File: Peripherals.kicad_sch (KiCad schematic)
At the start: 6 parts, among them J1 Conn_01x02, J4 Conn_02x10_Counter_Clockwise, Q1 PMOS, Q2 NMOS, U6 TPS62133

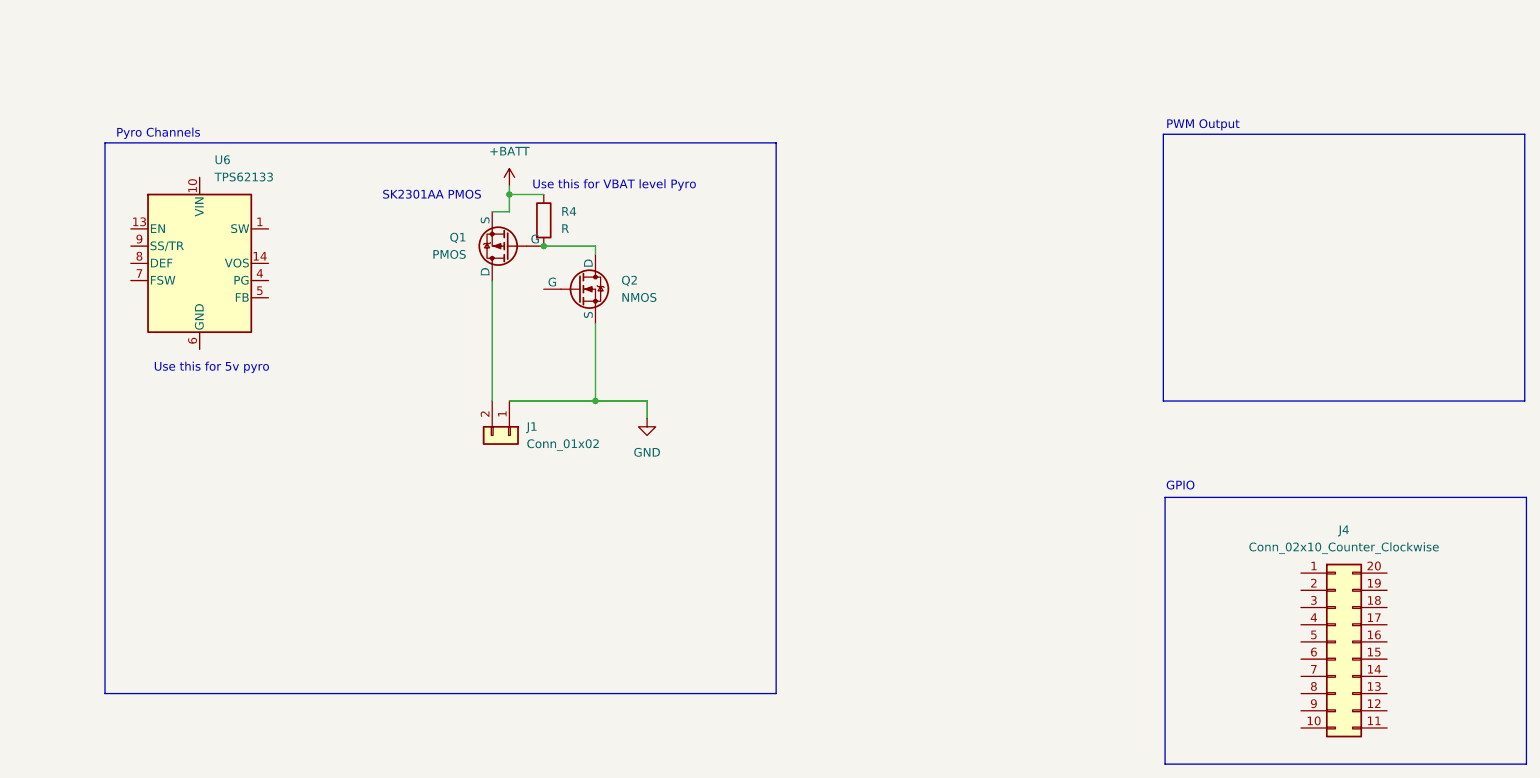
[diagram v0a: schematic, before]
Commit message: 5v⚡️
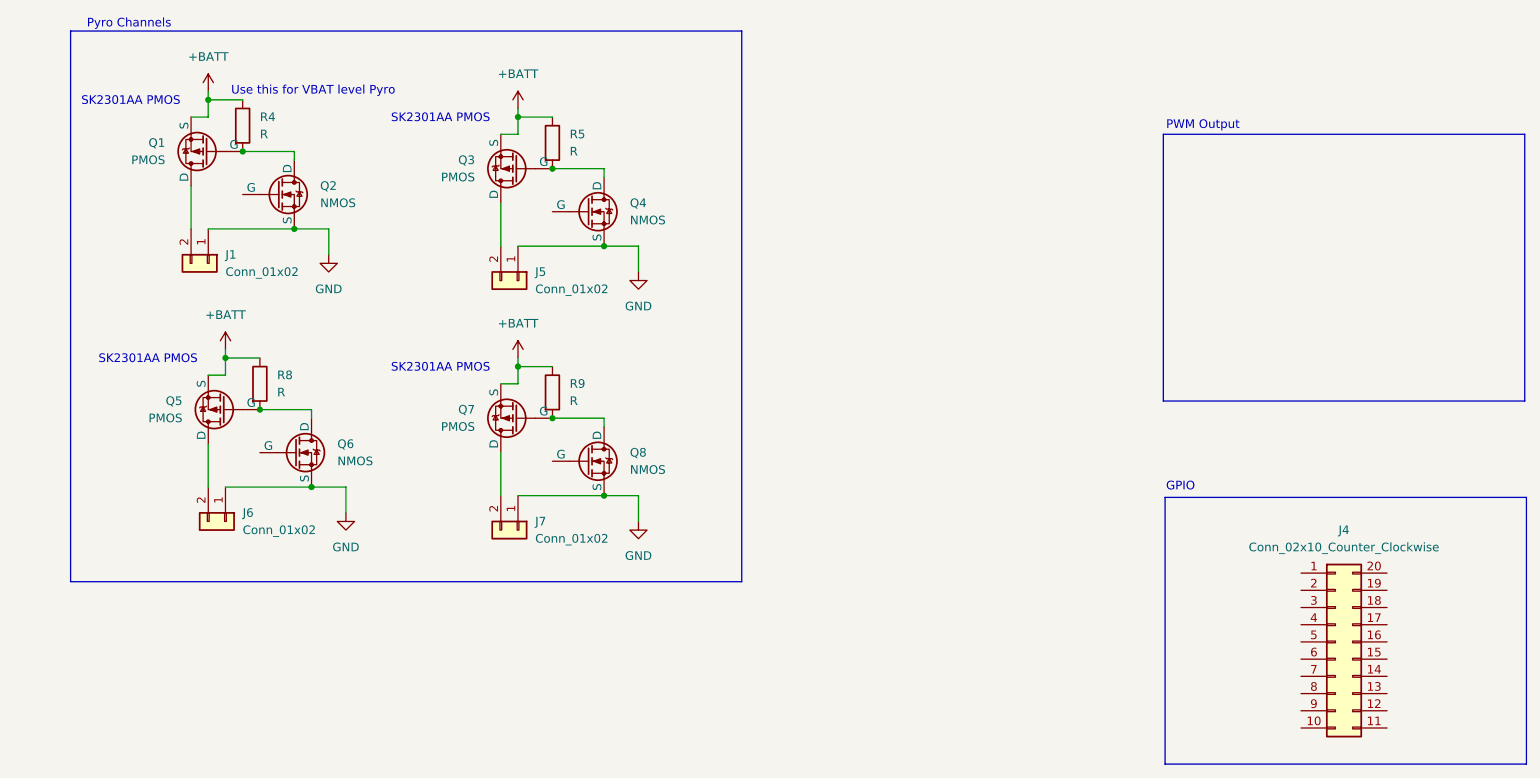
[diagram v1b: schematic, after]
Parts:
- removed U6: TPS62133, Package_DFN_QFN:VQFN-16-1EP_3x3mm_P0.5mm_EP1.68x1.68mm_ThermalVias, symbol Regulator_Switching:TPS62133
- added J5, J6, J7: Conn_01x02, symbol Connector_Generic:Conn_01x02
- added Q3, Q5, Q7: PMOS, symbol Simulation_SPICE:PMOS
- added Q4, Q6, Q8: NMOS, symbol Simulation_SPICE:NMOS
- added R5, R8, R9: R, 10k, symbol Device:R
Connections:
- net +BATT: now also Q3.3 (S), Q5.3 (S), Q7.3 (S), R5.1, R8.1, R9.1
- net GND: now also J5.1 (Pin_1), J6.1 (Pin_1), J7.1 (Pin_1), Q4.3 (S), Q6.3 (S), Q8.3 (S)
- new net: Q5.2 (G), Q6.1 (D), R8.2
- new net: J5.2 (Pin_2), Q3.1 (D)
- new net: Q3.2 (G), Q4.1 (D), R5.2
- new net: J7.2 (Pin_2), Q7.1 (D)
- new net: Q7.2 (G), Q8.1 (D), R9.2
- new net: J6.2 (Pin_2), Q5.1 (D)
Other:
- note removed: "Use this for 5v pyro"
- moved on the sheet: J1, Q1, Q2, R4

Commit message: FETS🦈
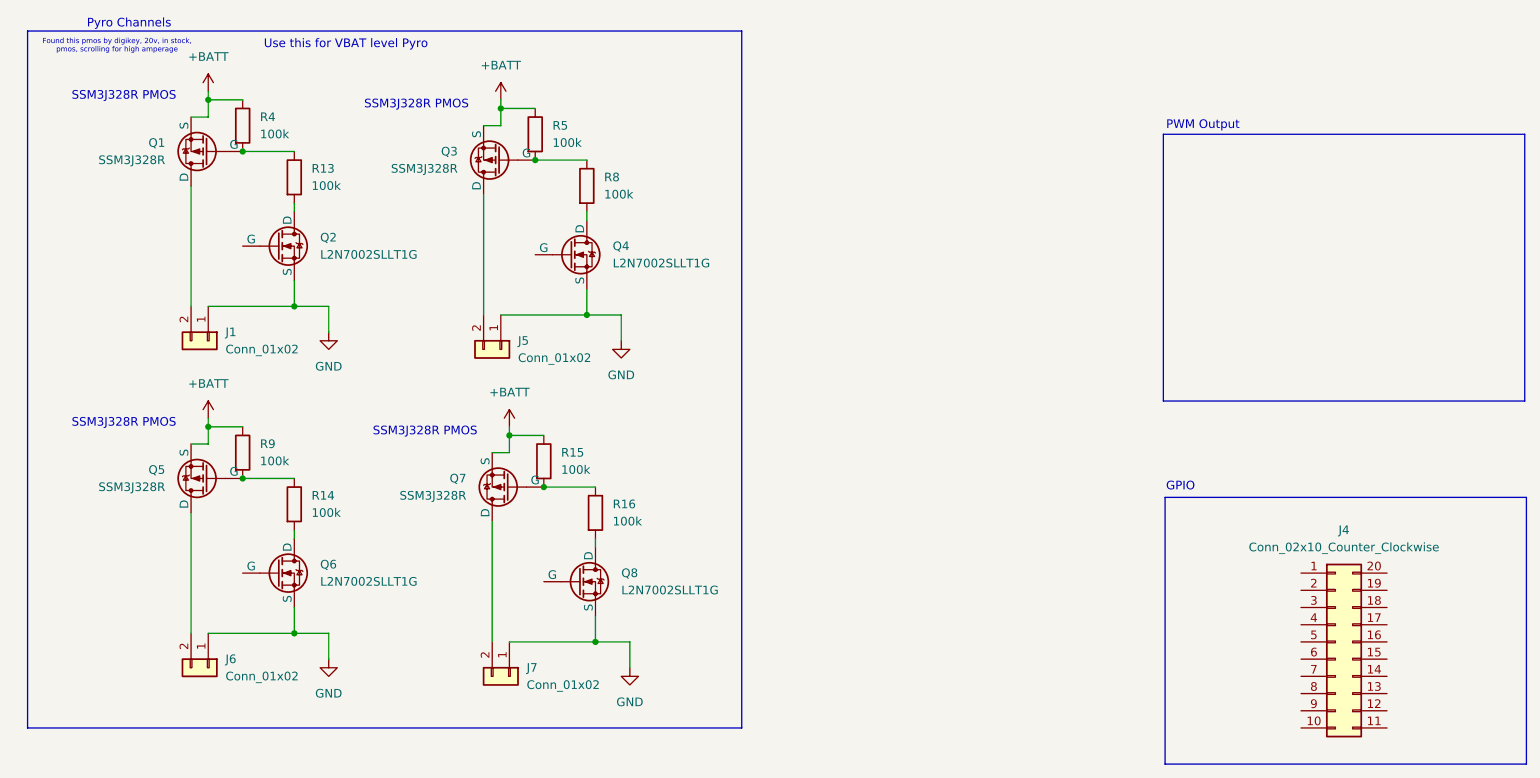
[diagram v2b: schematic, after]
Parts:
- added R13, R14, R15, R16: 100k, Resistor_SMD:R_0603_1608Metric, symbol Device:R
- Q1, Q3, Q5, Q7: value PMOS -> SSM3J328R; footprint (none) -> SSM3J328R:SOT95P240X88-3N
- Q2, Q4, Q6, Q8: value NMOS -> L2N7002SLLT1G; footprint (none) -> Package_TO_SOT_SMD:SOT-23
- R4, R5, R8, R9: value R -> 100k; footprint 10k -> Resistor_SMD:R_0603_1608Metric
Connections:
- net +BATT: now also R15.1; no longer R8.1
- net at Q3.2 (G), R5.2: now also R8.1; no longer Q4.1 (D)
- net at Q1.2 (G), R4.2: now also R13.1; no longer Q2.1 (D)
- new net: Q5.2 (G), R14.1, R9.2
- new net: Q4.1 (D), R8.2
- new net: Q6.1 (D), R14.2
- new net: Q2.1 (D), R13.2
- new net: Q7.2 (G), R15.2, R16.1
- new net: Q8.1 (D), R16.2
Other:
- note added: "Found this pmos by digikey, 20v, in stock, pmos, scrolling for high amperage"
- note added: "SSM3J328R PMOS"
- note removed: "SK2301AA PMOS"
- moved on the sheet: J1, Q2
